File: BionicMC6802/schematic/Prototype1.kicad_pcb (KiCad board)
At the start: 2 copper layers, 95 x 72 mm, 12 parts, among them SW1 TSD1265, U1 MC6802P, U2 74HCT541

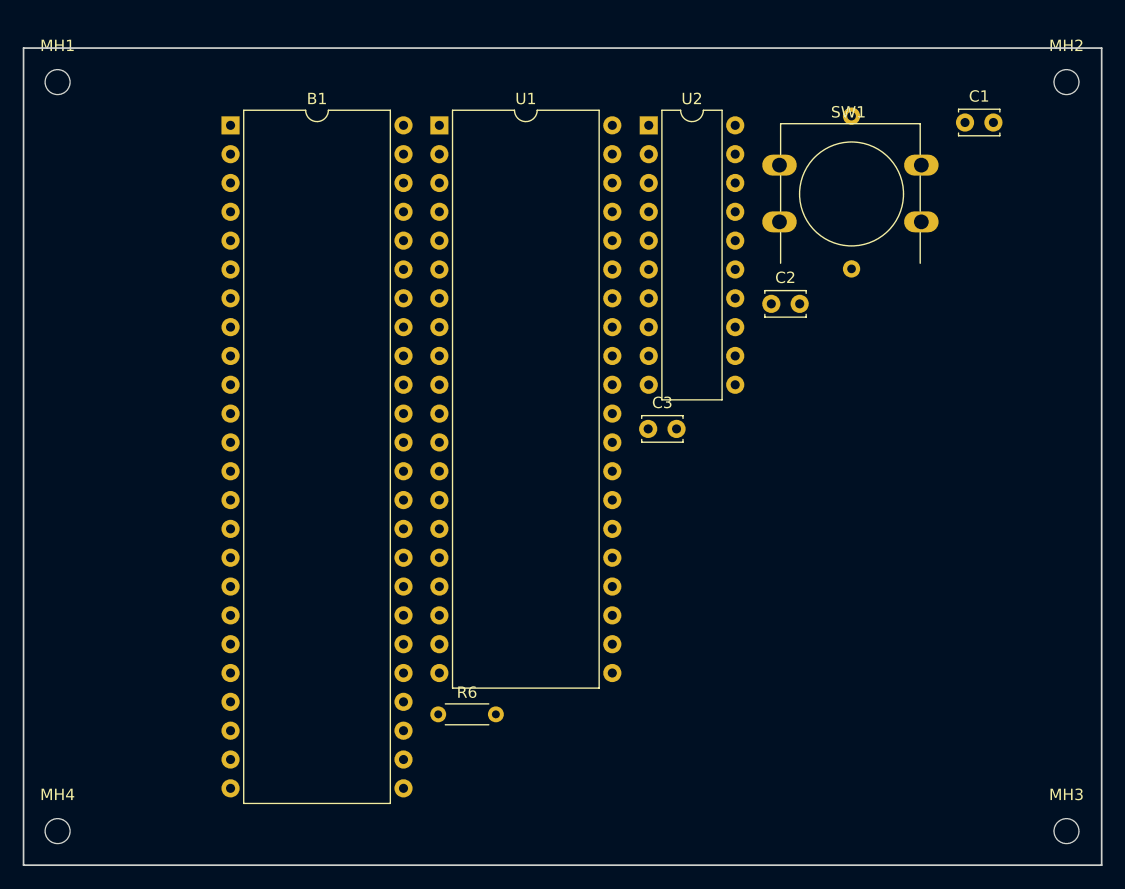
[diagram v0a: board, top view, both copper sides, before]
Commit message: [BionicMC6802] Mezzanine board
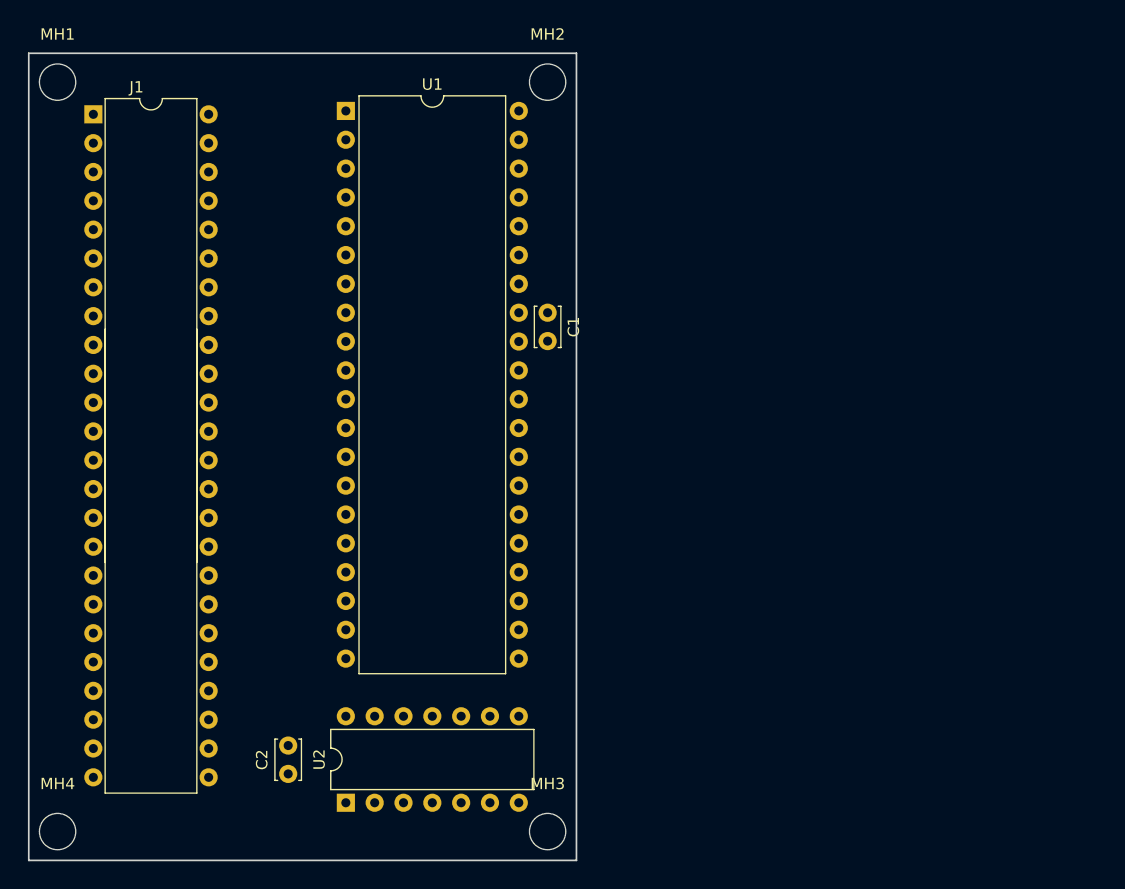
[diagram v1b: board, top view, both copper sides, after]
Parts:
- removed B1: Teensy3.5, Package_DIP:DIP-48_W15.24mm
- removed C3: 0.1u, Capacitor_THT:C_Disc_D3.4mm_W2.1mm_P2.50mm
- removed R6: 560, Resistor_THT:R_Axial_DIN0204_L3.6mm_D1.6mm_P5.08mm_Horizontal
- removed SW1: TSD1265, 0-LocalLibrary:SW_PUSH-LED-12mm
- added J1: BionicConnector, 0-LocalLibrary:DIP-48_W10.16mm, F.Cu at (104.2, 72.8)
- MH1, MH2, MH3, MH4: value MountingHole_2.2mm_M2 -> MountingHole_3.2mm_M3; footprint MountingHole:MountingHole_2.2mm_M2 -> MountingHole:MountingHole_3.2mm_M3
- U2: value 74HCT541 -> 74HCT126; footprint Package_DIP:DIP-20_W7.62mm -> Package_DIP:DIP-14_W7.62mm
- moved U2 65.4 mm to (126.4, 133.5), turned to 90 degrees
- moved C2 59.4 mm to (121.3, 131.0), turned to 90 degrees
- moved MH3 45.7 mm to (144.2, 136.0)
- moved MH2 45.7 mm to (144.2, 70.0)
- moved C1 40.4 mm to (144.2, 90.3), turned to 270 degrees
- moved U1 8.34 mm to (126.4, 72.5)
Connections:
- U1 pad 10: /A1 -> /P21
- U1 pad 11: /A2 -> /P22
- U1 pad 12: /A3 -> /P23
- U1 pad 13: /A4 -> /P24
- U1 pad 14: /A5 -> /P25
- U1 pad 15: /A6 -> /P26
- U1 pad 16: /A7 -> /P27
- U1 pad 17: /A8 -> /P30
- U1 pad 18: /A9 -> /P31
- U1 pad 19: /A10 -> /P32
- U1 pad 2: /~HALT~ -> /P40
- U1 pad 20: /A11 -> /P33
- U1 pad 22: /A12 -> /P34
- U1 pad 23: /A13 -> /P35
- U1 pad 24: /A14 -> /P36
- U1 pad 25: /A15 -> /P37
- U1 pad 26: /D7 -> /P17
- U1 pad 27: /D6 -> /P16
- U1 pad 28: /D5 -> /P15
- U1 pad 29: /D4 -> /P14
- U1 pad 3: /MR -> /P52
- U1 pad 30: /D3 -> /P13
- U1 pad 31: /D2 -> /P12
- U1 pad 32: /D1 -> /P11
- U1 pad 33: /D0 -> /P10
- U1 pad 34: /R~W~ -> /P41
- U1 pad 36: GND -> /P51
- U1 pad 37: /CLK_E -> /P47
- U1 pad 39: Net-(R1-Pad1) -> /P46
- U1 pad 4: /~IRQ~ -> /P42
- U1 pad 40: /~RESET~ -> /#RESET
- U1 pad 5: /VMA -> /P50
- U1 pad 6: /~NMI~ -> /P43
- U1 pad 7: /BA -> /P55
- U1 pad 9: /A0 -> /P20
- U2 pad 1: GND -> VCC
- U2 pad 12: Net-(U2-Pad12) -> GND
- U2 pad 13: Net-(U2-Pad13) -> GND
- U2 pad 14: Net-(U2-Pad14) -> VCC
- U2 pad 2: Net-(B1-Pad21) -> /P53
- U2 pad 3: Net-(B1-Pad17) -> /#RESET
- U2 pad 6: GND -> Net-(U2-Pad6)
- U2 pad 8: GND -> Net-(U2-Pad8)
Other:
- board size 95 x 72 mm -> 48.3 x 71.1 mm
